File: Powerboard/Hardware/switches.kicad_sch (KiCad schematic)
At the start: 26 parts, among them J2 FAN, J4 Conn_01x02_Male, J5 Conn_01x08_Male, J6 Conn_01x02_Male, Q1 SSM3K15AMFV,L3F, Q10 SQS141ELNW-T1_GE3, Q7 SQS141ELNW-T1_GE3, Q8 SQS141ELNW-T1_GE3, Q9 SQS141ELNW-T1_GE3, U6 LTC4412xS6, U7 LTC4412xS6

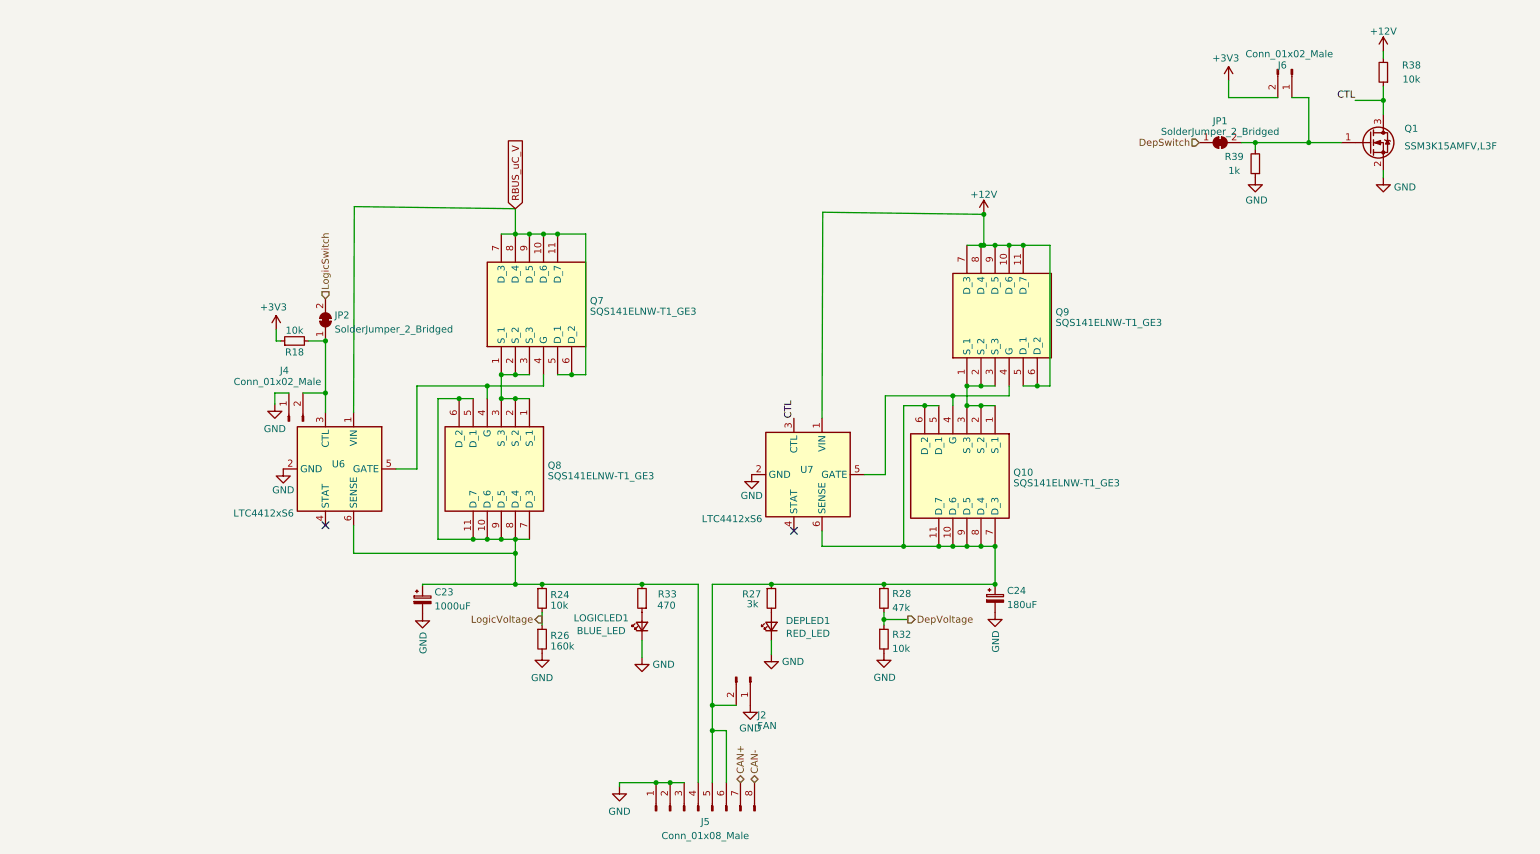
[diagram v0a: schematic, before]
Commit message: shiven layout change
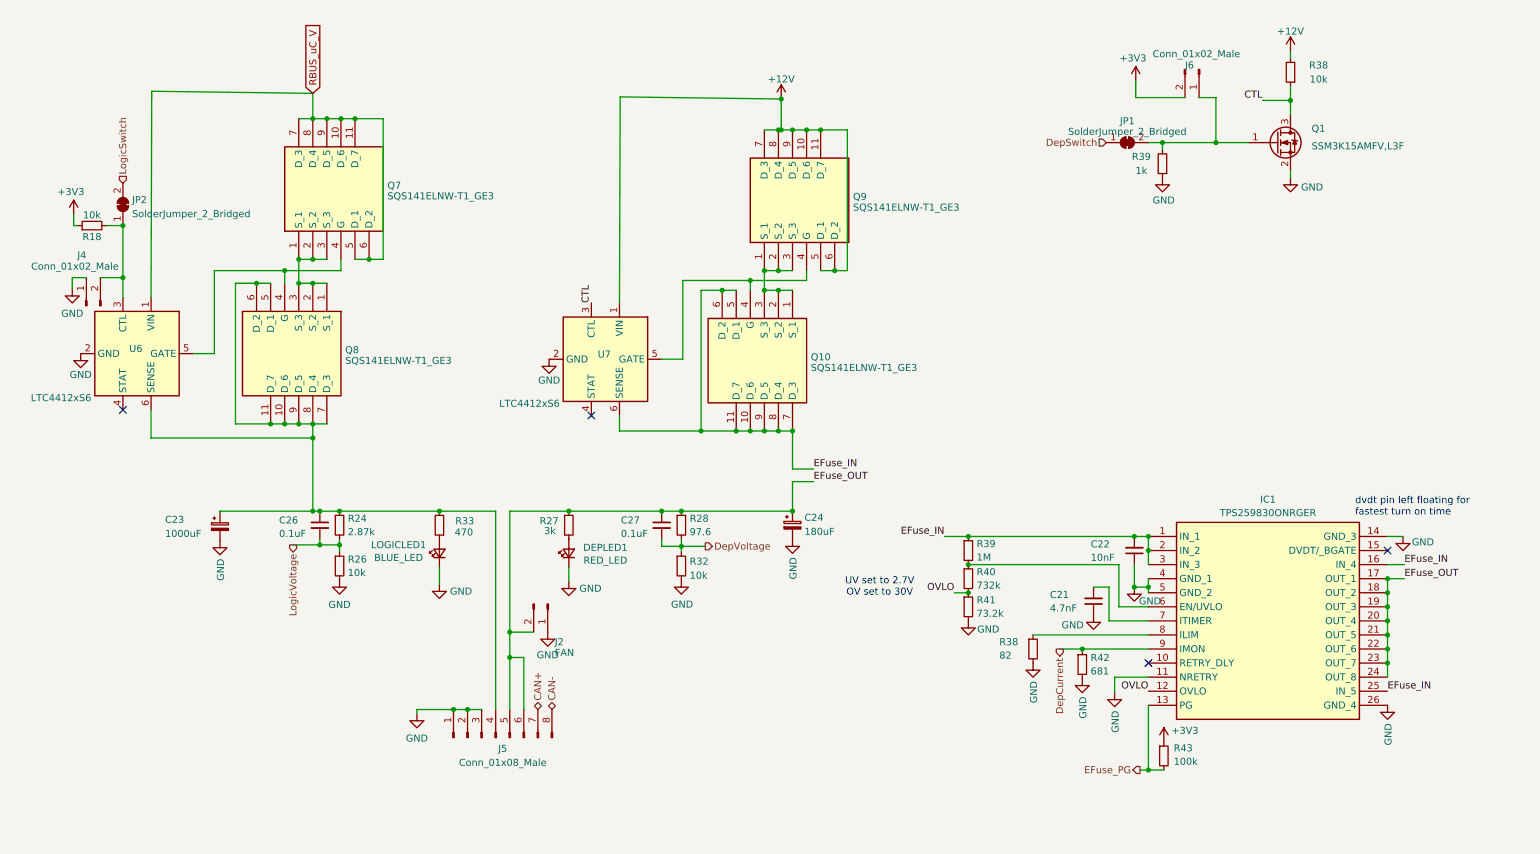
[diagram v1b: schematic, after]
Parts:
- added C21: 4.7nF, Capacitor_SMD:C_0402_1005Metric, symbol Device:C_Small
- added C22: 10nF, Capacitor_SMD:C_0402_1005Metric, symbol Device:C_Small
- added C26, C27: 0.1uF, Capacitor_SMD:C_0402_1005Metric, symbol Device:C_Small
- added IC1: TPS259830ONRGER, iclr:TPS259830ONRGER, symbol iclr:TPS259830ONRGER
- added R38: 82, Capacitor_SMD:C_0402_1005Metric, symbol Device:R_Small
- added R39: 1M, Capacitor_SMD:C_0402_1005Metric, symbol Device:R_Small
- added R40: 732k, Capacitor_SMD:C_0402_1005Metric, symbol Device:R_Small
- added R41: 73.2k, Capacitor_SMD:C_0402_1005Metric, symbol Device:R_Small
- added R42: 681, Capacitor_SMD:C_0402_1005Metric, symbol Device:R_Small
- added R43: 100k, Capacitor_SMD:C_0402_1005Metric, symbol Device:R_Small
- R24: value 10k -> 2.87k
- R26: value 160k -> 10k
- R28: value 47k -> 97.6
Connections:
- net +3V3: now also R43.1
- net DepVoltage: now also C27.2
- net GND: now also C21.1, C22.1, IC1.11 (NRETRY), IC1.14 (GND_3), IC1.26 (GND_4), IC1.4 (GND_1), IC1.5 (GND_2), R38.2, R41.2, R42.2
- net LogicVoltage: now also C26.2
- net at C23.1, J5.4 (Pin_4), Q8.10 (D_6)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: now also C26.1
- net EFuse_IN: now reaches Q10.10 (D_6), Q10.11 (D_7), Q10.5 (D_1), Q10.6 (D_2), Q10.7 (D_3), Q10.8 (D_4), Q10.9 (D_5), U7.6 (SENSE)
- net EFuse_IN: now also C22.2, IC1.1 (IN_1), IC1.16 (IN_4), IC1.2 (IN_2), IC1.25 (IN_5), IC1.3 (IN_3), R39.1; no longer C24.1, J2.2 (Pin_2), J5.5 (Pin_5), J5.6 (Pin_6), R27.1, R28.1
- new net: IC1.8 (ILIM), R38.1
- new net: C21.2, IC1.7 (ITIMER)
- new net: IC1.6 (EN/UVLO), R39.2, R40.1
- new net DepCurrent: IC1.9 (IMON), R42.1
- new net EFuse_OUT: C24.1, C27.1, IC1.17 (OUT_1), IC1.18 (OUT_2), IC1.19 (OUT_3), IC1.20 (OUT_4), IC1.21 (OUT_5), IC1.22 (OUT_6), IC1.23 (OUT_7), IC1.24 (OUT_8), J2.2 (Pin_2), J5.5 (Pin_5), J5.6 (Pin_6), R27.1, R28.1
- new net EFuse_PG: IC1.13 (PG), R43.2
- new net OVLO: IC1.12 (OVLO), R40.2, R41.1
- no-connect marks 2 -> 4
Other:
- note added: "UV set to 2.7V OV set to 30V"
- note added: "dvdt pin left floating for fastest turn on time"
- moved on the sheet: C23, C24, DEPLED1, J2, J4, J5, J6, JP1, JP2, LOGICLED1, Q1, Q10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
